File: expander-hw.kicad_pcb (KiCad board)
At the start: 2 copper layers, 15 parts, among them J1 Conn_ARM_JTAG_SWD_10, J2 USB_C_Receptacle_USB2.0_16P, J3 Conn_02x08_Odd_Even, U1 STM32H562RGTx, U2 SRDA3.3-4BTG, U3 AZ1117-3.3, U4 SRDA3.3-4BTG, U5 USBLC6-2SC6, U6 SRDA3.3-4BTG

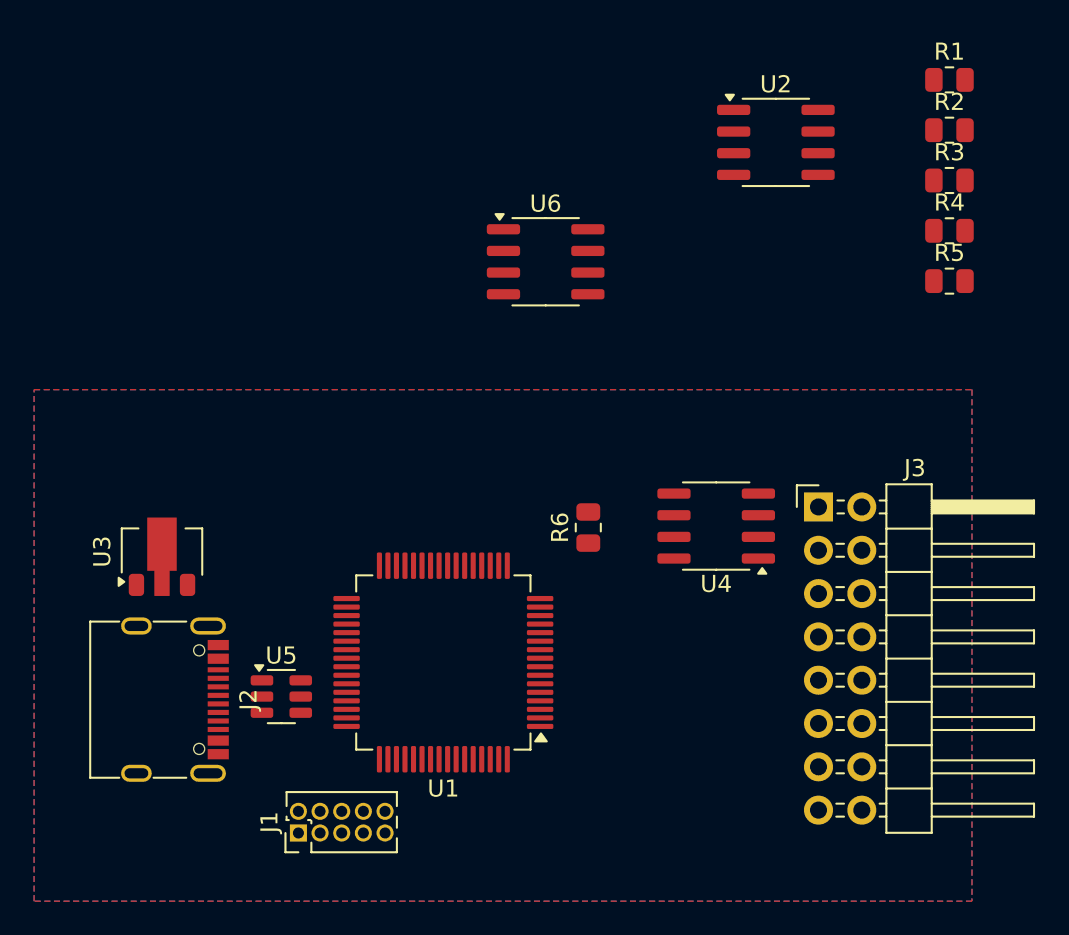
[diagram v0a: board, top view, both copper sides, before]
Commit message: save
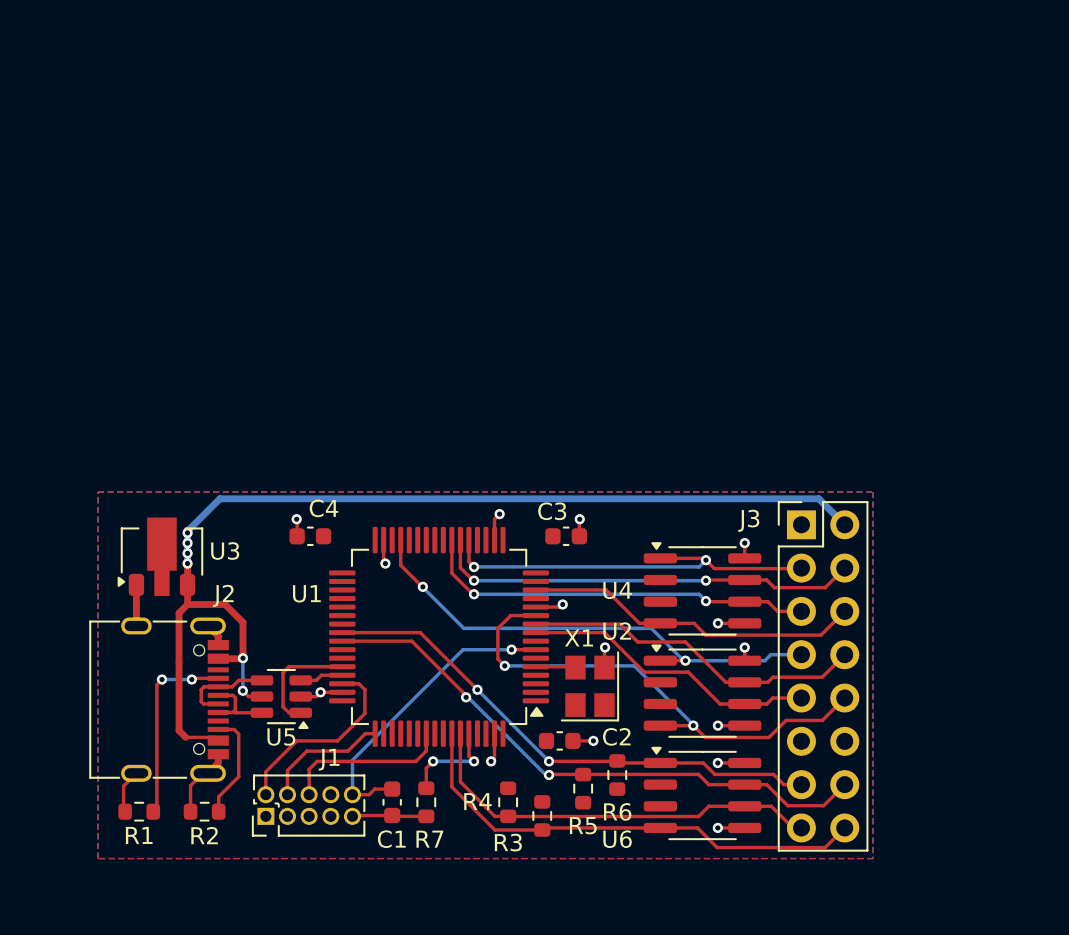
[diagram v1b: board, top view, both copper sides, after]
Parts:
- added C1: 100nF, Capacitor_SMD:C_0603_1608Metric, F.Cu at (126.0, 109.2)
- added C2: 100nF, Capacitor_SMD:C_0603_1608Metric, F.Cu at (135.8, 105.6)
- added C3: 100nF, Capacitor_SMD:C_0603_1608Metric, F.Cu at (136.2, 93.6)
- added C4: 100nF, Capacitor_SMD:C_0603_1608Metric, F.Cu at (121.2, 93.6)
- added R7: 10k, Resistor_SMD:R_0603_1608Metric, F.Cu at (128.0, 109.2)
- added X1: ECS-2520MV-xxx-xx, Crystal:Crystal_SMD_TXC_7M-4Pin_3.2x2.5mm, F.Cu at (137.6, 102.4)
- J3: footprint Connector_PinHeader_2.54mm:PinHeader_2x08_P2.54mm_Horizontal -> Connector_PinHeader_2.54mm:PinHeader_2x08_P2.54mm_Vertical
- R1, R2, R3, R4, R5, R6: footprint Resistor_SMD:R_0805_2012Metric -> Resistor_SMD:R_0603_1608Metric
- moved R1 64.0 mm to (111.2, 109.8), turned to 180 degrees
- moved R2 59.2 mm to (115.0, 109.8), turned to 180 degrees
- moved R3 44.3 mm to (134.8, 110.0), turned to -90 degrees
- moved R4 42.3 mm to (132.8, 109.2), turned to -90 degrees
- moved R5 36.7 mm to (137.2, 108.4), turned to 90 degrees
- moved U6 32.6 mm to (144.2, 108.8)
- moved U2 32.6 mm to (144.2, 102.8)
- moved R6 14.6 mm to (139.2, 107.6)
- moved U4 3.88 mm to (144.2, 96.8), turned to 0 degrees
- moved J1 2.14 mm to (118.6, 110.0)
- moved U1 1.52 mm to (128.8, 99.5)
- moved J3 1.45 mm to (150.0, 92.9)
- turned U5 to 180 degrees
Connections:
- J3 pad 1: /I2C1_SDA -> +3.3V
- J3 pad 10: unconnected-(J3-Pin_10-Pad10) -> /SPI2_CS
- J3 pad 11: unconnected-(J3-Pin_11-Pad11) -> GND
- J3 pad 12: unconnected-(J3-Pin_12-Pad12) -> GND
- J3 pad 13: unconnected-(J3-Pin_13-Pad13) -> /I2C3_SDA
- J3 pad 14: unconnected-(J3-Pin_14-Pad14) -> /I2C3_SCL
- J3 pad 15: unconnected-(J3-Pin_15-Pad15) -> /I2C1_SDA
- J3 pad 16: unconnected-(J3-Pin_16-Pad16) -> /I2C1_SCL
- J3 pad 2: /I2C3_SDA -> VBUS
- J3 pad 3: /I2C1_SCL -> /SPI1_SCK
- J3 pad 4: /I2C3_SCL -> /SPI1_MISO
- J3 pad 5: GND -> /SPI1_MOSI
- J3 pad 6: +3.3V -> /SPI1_CS
- J3 pad 7: GND -> /SPI2_SCK
- J3 pad 8: VBUS -> /SPI2_MISO
- J3 pad 9: unconnected-(J3-Pin_9-Pad9) -> /SPI2_MOSI
- R3 pad 2: Net-(U4-I/O1) -> /I2C1_SCL
- R4 pad 2: Net-(U4-I/O2) -> /I2C1_SDA
- R5 pad 2: Net-(U4-I/O3) -> /I2C3_SCL
- R6 pad 2: Net-(U4-I/O4) -> /I2C3_SDA
- U1 pad 10: unconnected-(U1-PC2-Pad10) -> /SPI2_MISO
- U1 pad 11: unconnected-(U1-PC3-Pad11) -> /SPI2_CS
- U1 pad 14: unconnected-(U1-PA0-Pad14) -> /SPI1_CS
- U1 pad 21: unconnected-(U1-PA5-Pad21) -> /SPI1_SCK
- U1 pad 22: unconnected-(U1-PA6-Pad22) -> /SPI1_MISO
- U1 pad 23: unconnected-(U1-PA7-Pad23) -> /SPI1_MOSI
- U1 pad 29: /I2C2_SCL -> /SPI2_SCK
- U1 pad 33: /I2C2_SDA -> unconnected-(U1-PB12-Pad33)
- U1 pad 5: unconnected-(U1-PH0-Pad5) -> /PH0
- U1 pad 6: unconnected-(U1-PH1-Pad6) -> /PH1
- U1 pad 60: unconnected-(U1-BOOT0-Pad60) -> Net-(U1-BOOT0)
- U1 pad 7: unconnected-(U1-NRST-Pad7) -> /~{RESET}
- U1 pad 9: unconnected-(U1-PC1-Pad9) -> /SPI2_MOSI
- U2 pad 1: unconnected-(U2-I/O1-Pad1) -> /SPI2_SCK
- U2 pad 4: unconnected-(U2-I/O2-Pad4) -> /SPI2_CS
- U2 pad 6: unconnected-(U2-I/O3-Pad6) -> /SPI2_MOSI
- U2 pad 7: unconnected-(U2-I/O4-Pad7) -> /SPI2_MISO
- U4 pad 1: Net-(U4-I/O1) -> /SPI1_SCK
- U4 pad 4: Net-(U4-I/O2) -> /SPI1_CS
- U4 pad 6: Net-(U4-I/O3) -> /SPI1_MOSI
- U4 pad 7: Net-(U4-I/O4) -> /SPI1_MISO
- U5 pad 1: Net-(J2-D--PadA7) -> /D-
- U5 pad 3: Net-(J2-D+-PadA6) -> /D+
- U5 pad 4: /D- -> Net-(J2-D--PadA7)
- U5 pad 6: /D+ -> Net-(J2-D+-PadA6)
- U6 pad 1: unconnected-(U6-I/O1-Pad1) -> /I2C3_SDA
- U6 pad 4: unconnected-(U6-I/O2-Pad4) -> /I2C1_SCL
- U6 pad 6: unconnected-(U6-I/O3-Pad6) -> /I2C1_SDA
- U6 pad 7: unconnected-(U6-I/O4-Pad7) -> /I2C3_SCL
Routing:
- net VBUS: track 0.00 -> 64.9 mm, vias 0 -> 6
- net GND: track 0.00 -> 37.1 mm, vias 0 -> 15
- net /I2C3_SCL: track 0.00 -> 34.1 mm, vias 0 -> 2
- net /I2C3_SDA: track 0.00 -> 30.6 mm, vias 0 -> 2
- net /SPI2_CS: track 0.00 -> 29.5 mm, vias 0 -> 2
- net /SPI2_SCK: track 0.00 -> 29.1 mm, vias 0 -> 2
- net /I2C1_SCL: track 0.00 -> 28.2 mm
- net /SPI1_MISO: track 0.00 -> 25.2 mm, vias 0 -> 2
- net /I2C1_SDA: track 0.00 -> 24.4 mm
- net /SPI1_SCK: track 0.00 -> 24.0 mm, vias 0 -> 2
- net /SPI1_MOSI: track 0.00 -> 23.4 mm, vias 0 -> 2
- net /SPI2_MISO: track 0.00 -> 20.2 mm
- net /SPI1_CS: track 0.00 -> 19.8 mm
- net /~{RESET}: track 0.00 -> 17.9 mm, vias 0 -> 1
- net /SPI2_MOSI: track 0.00 -> 17.5 mm
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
